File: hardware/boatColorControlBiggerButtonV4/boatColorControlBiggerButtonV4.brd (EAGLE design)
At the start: 125.7 x 98.4 mm, 48 parts

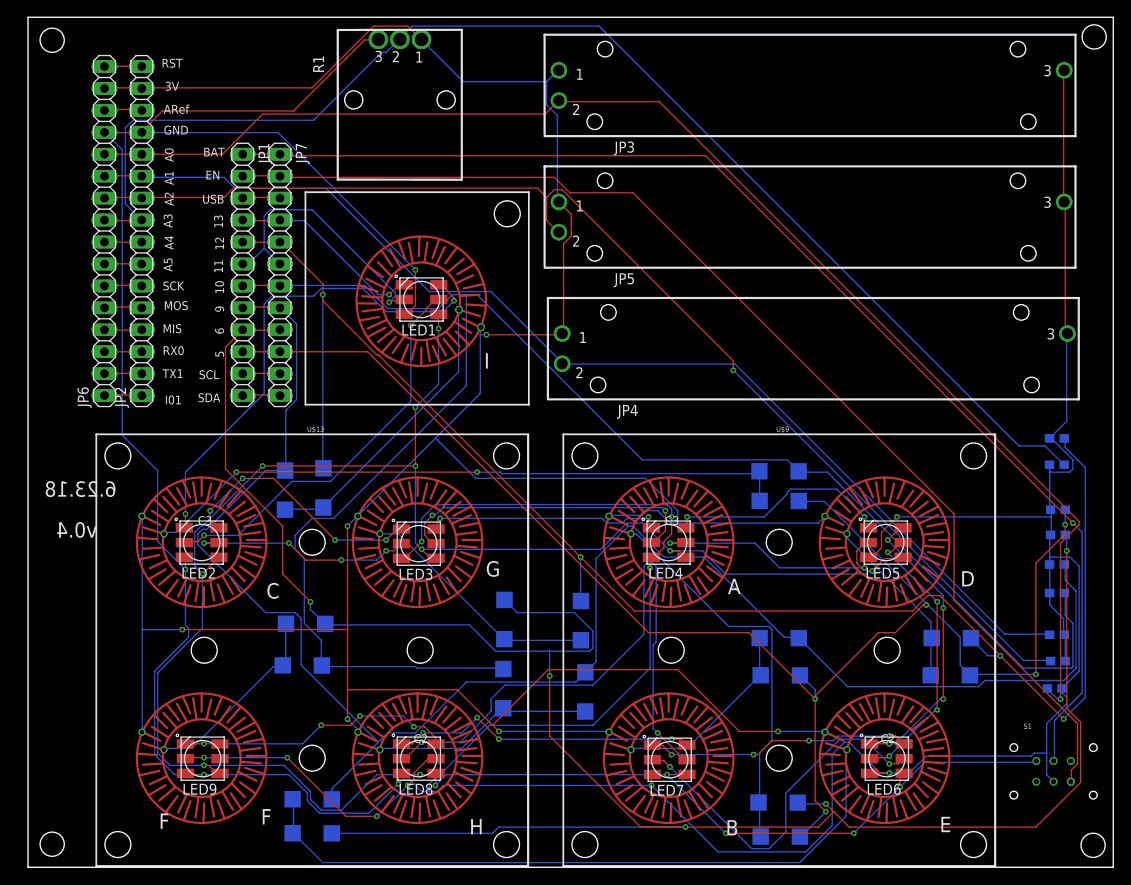
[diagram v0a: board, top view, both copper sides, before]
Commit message: hardware update
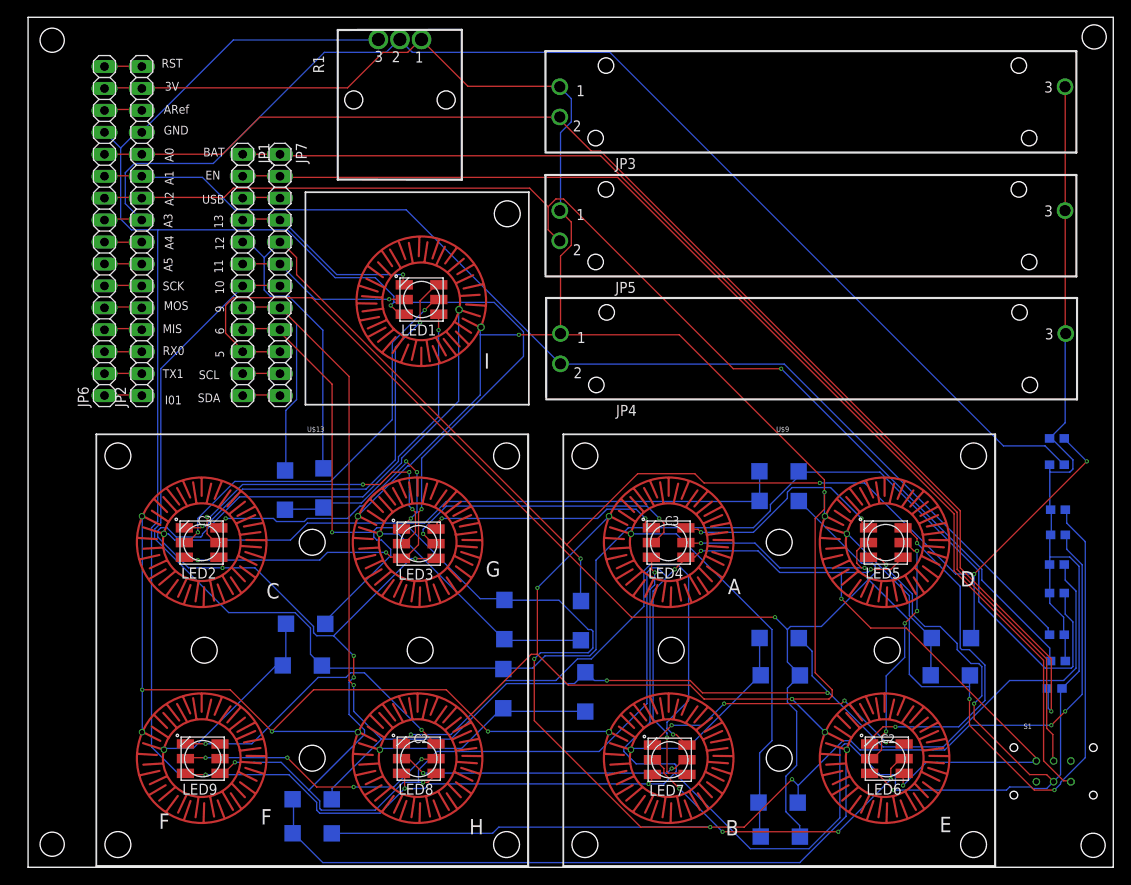
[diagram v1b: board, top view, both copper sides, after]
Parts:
- moved JP3 1.90 mm to (61.6, 86.9)
- moved JP5 1.00 mm to (61.6, 72.5)
- moved JP4 0.20 mm to (61.6, 58.3)
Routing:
- net PIN5: track 180.1 -> 218.5 mm, vias 5 -> 3
- net N$13: track 69.1 -> 34.4 mm
- net N$12: track 35.6 -> 66.6 mm, vias 4 -> 2
- net LEDPWR: track 273.9 -> 304.6 mm, vias 15 -> 13
- net PWR: track 337.5 -> 359.0 mm, vias 6 -> 7
- net GND: track 509.4 -> 529.8 mm, vias 10 -> 11
- net N$7: track 26.2 -> 38.8 mm
- net PIN11: track 32.3 -> 20.4 mm
- net PIN10: track 200.0 -> 189.1 mm
- net BAT: track 143.2 -> 133.4 mm, vias 1 -> 0
- net PIN12: track 184.6 -> 175.5 mm
- net A0: track 159.2 -> 150.4 mm
- net N$4: track 57.0 -> 50.2 mm
- net N$10: track 34.1 -> 40.5 mm, vias 4 -> 2
- net PIN6: track 244.8 -> 239.1 mm, vias 5 -> 6
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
